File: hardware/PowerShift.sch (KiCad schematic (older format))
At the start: 46 parts, among them J1 Barrel_Jack, J10 SHIFT_OUT, J11 JST-ZR, J12 JST-ZR, J14 JST-ZR, J2 MICRO_USB, J3 JST-ZR, J4 JST-ZR, J5 SHIFT_IN, J6 SHIFT_IN, J7 AVR-PDI-6A, J8 JST-ZR, J9 JST-ZR, U1 MCP1700, U2 TPIC6B595, U3 TPIC6B595, U4 TPIC6B595, U5 TPIC6B595, U6 KT3225T, U7 TPIC6B595, U8 TPIC6B595, U9 ATXMEGA32E5-AU, Y1 Crystal

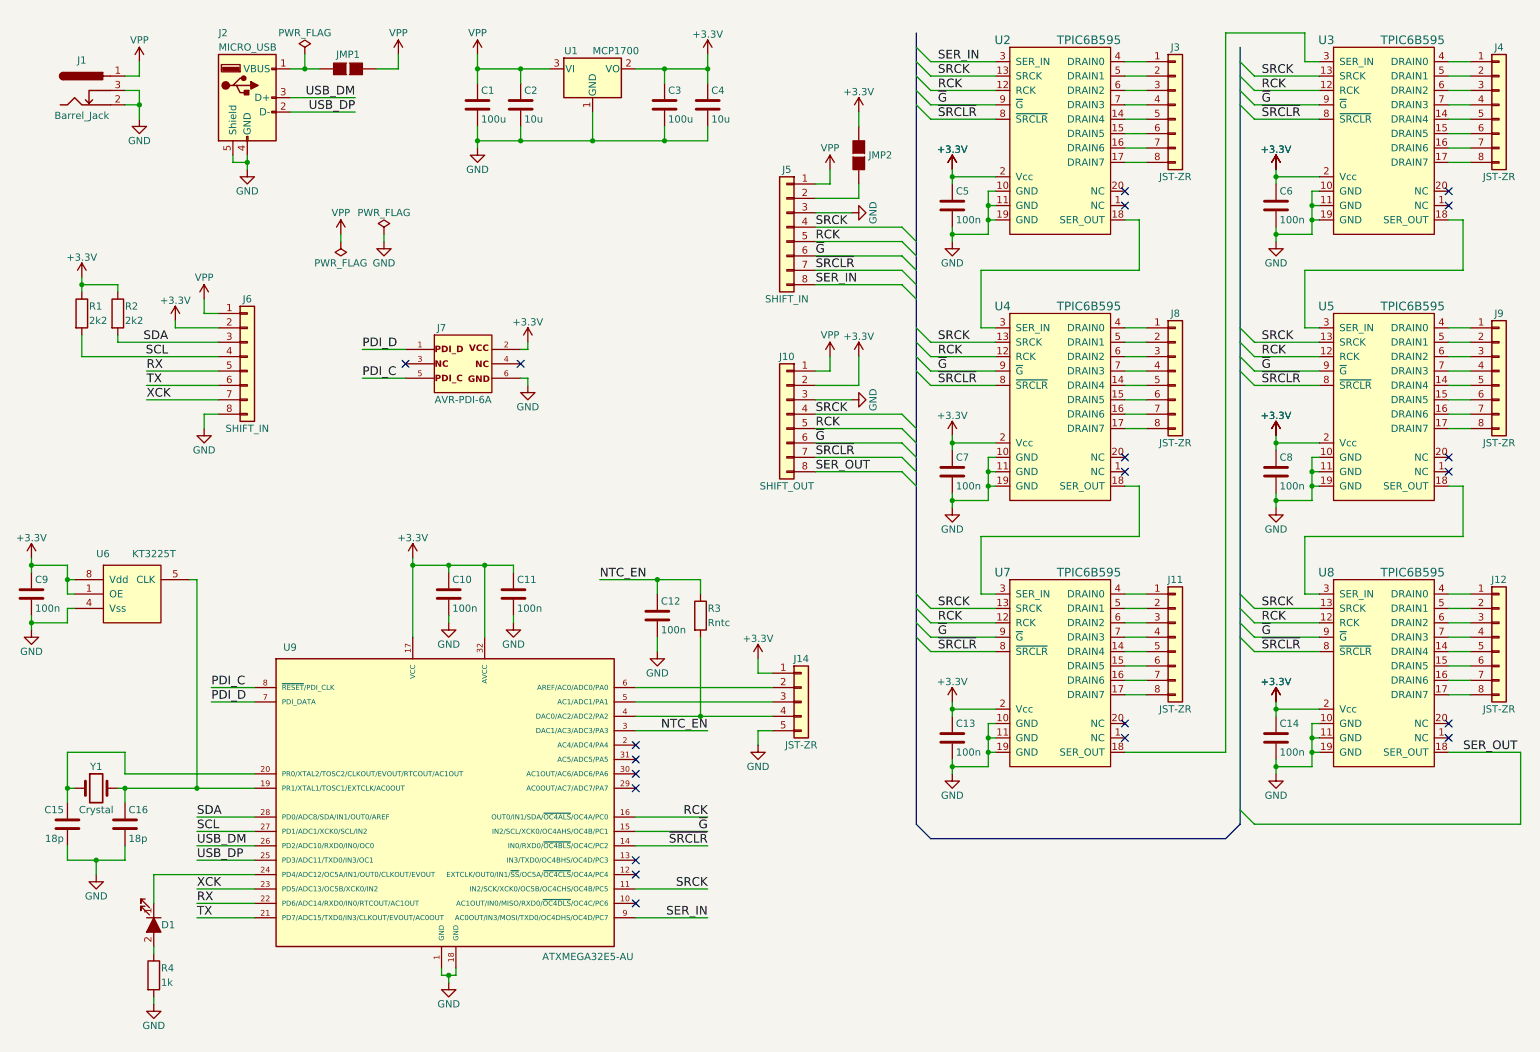
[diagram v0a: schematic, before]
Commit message: Step down regulator
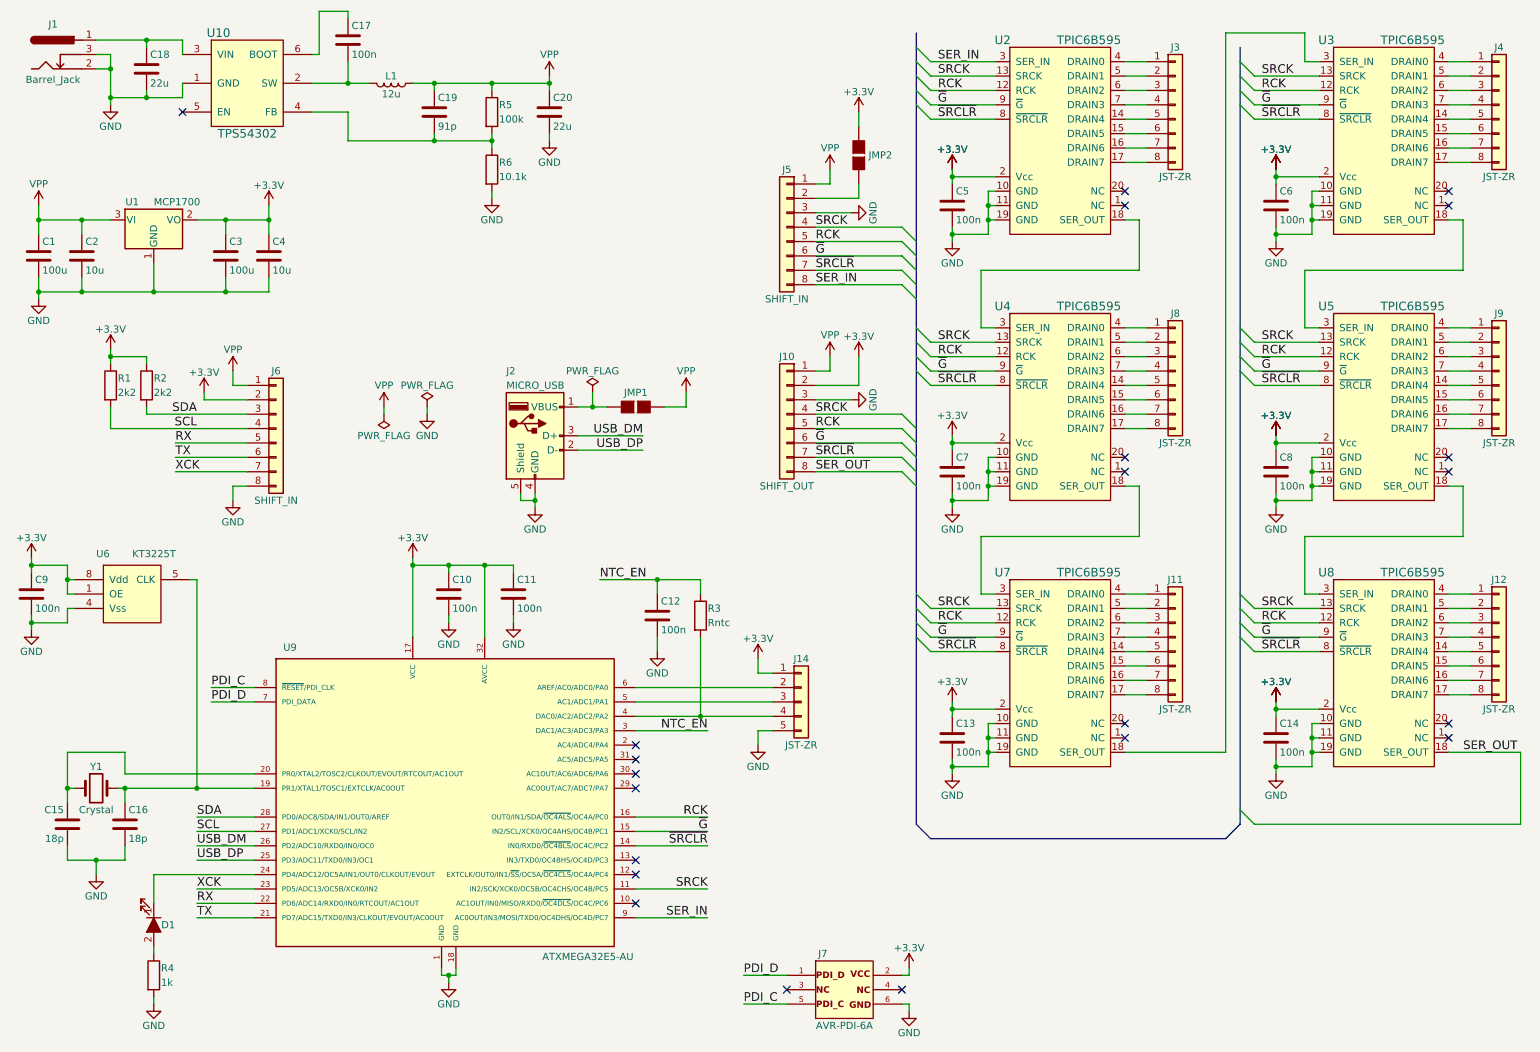
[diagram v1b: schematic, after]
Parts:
- added C17: 100n, symbol C
- added C18, C20: 22u, symbol C
- added C19: 91p, symbol C
- added L1: 12u, kuro:Bourns_SDR1307_14x14mm, symbol L
- added R5: 100k, symbol R
- added R6: 10.1k, symbol R
- added U10: TPS54302, symbol TPS54302
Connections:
- net GND: now also C18.2, C20.2, R6.2, U10.1 (GND)
- net VPP: now also C19.1, C20.1, L1.1, R5.1; no longer J1.1
- new net: C18.1, J1.1, U10.3 (VIN)
- new net: C17.2, L1.2, U10.2 (SW)
- new net: C19.2, R5.2, R6.1, U10.4 (FB)
- new net: C17.1, U10.6 (BOOT)
- no-connect marks 21 -> 22
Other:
- moved on the sheet: C1, C2, C3, C4, J1, J2, J6, J7, JMP1, R1, R2, U1
